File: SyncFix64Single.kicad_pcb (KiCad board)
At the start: 2 copper layers, 27.9 x 12.7 mm, 15 parts, among them J1 PWR, J2 Video, Q1 BSS138, Q2 BSS138, U1 LM1881, U2 AMS1117-50

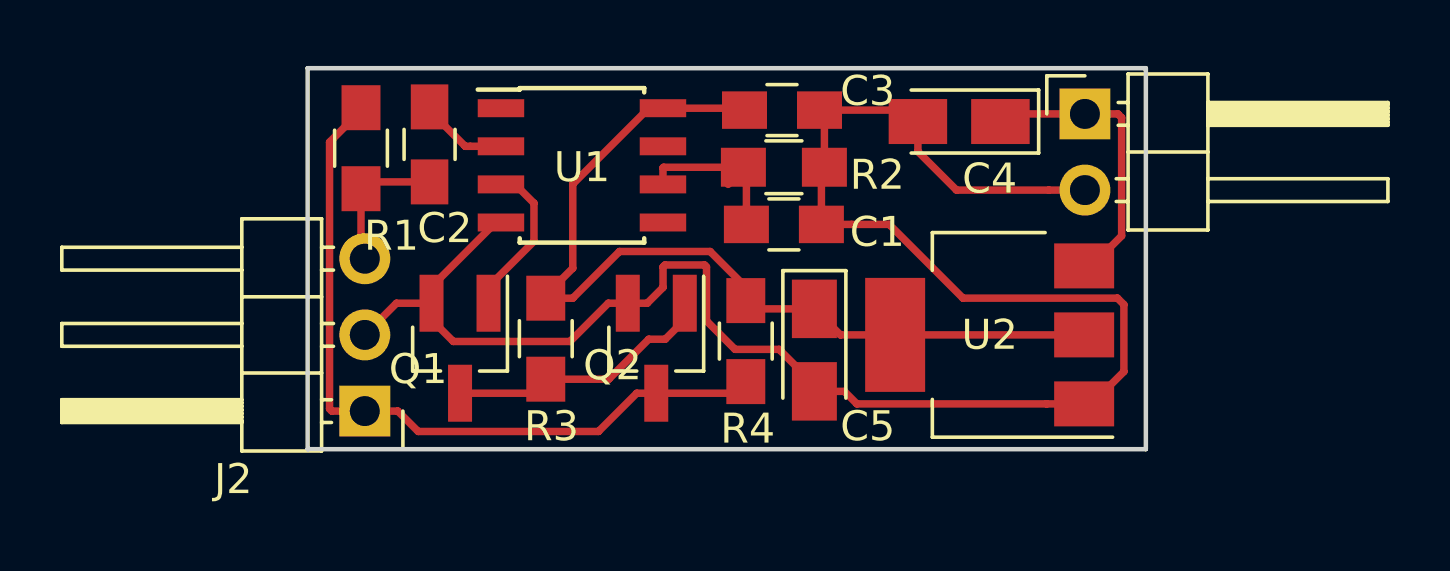
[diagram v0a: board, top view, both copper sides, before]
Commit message: Minor fixes.
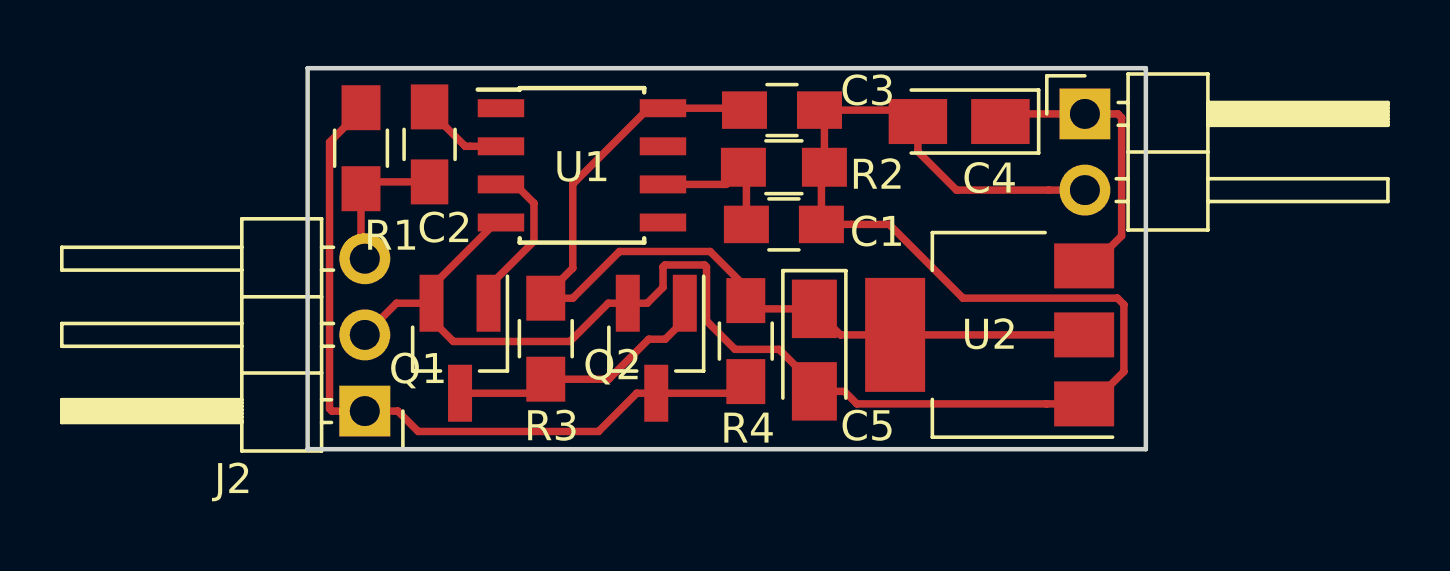
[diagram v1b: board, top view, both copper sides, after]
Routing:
- net Net-(C1-Pad1): track 5.96 -> 5.01 mm
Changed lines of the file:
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@@
     (thickness 1.6)
     (drawings 6)
-    (tracks 108)
+    (tracks 106)
     (zones 0)
     (modules 15)
@@
   (gr_line (start 57.15 27.94) (end 57.15 40.64) (angle 90) (layer Edge.Cuts) (width 0.15))
   (gr_line (start 29.21 27.94) (end 29.21 40.64) (angle 90) (layer Edge.Cuts) (width 0.15))
-  (segment (start 43.735 31.242) (end 41.0755 31.242) (width 0.25) (layer F.Cu) (net 1))
-  (segment (start 41.0755 31.242) (end 41.054 31.2635) (width 0.25) (layer F.Cu) (net 1))
-  (segment (start 41.054 31.2635) (end 41.054 31.8135) (width 0.25) (layer F.Cu) (net 1))
+  (segment (start 41.054 31.8135) (end 43.1635 31.8135) (width 0.25) (layer F.Cu) (net 1))
+  (segment (start 43.1635 31.8135) (end 43.735 31.242) (width 0.25) (layer F.Cu) (net 1))
   (segment (start 43.835 33.147) (end 43.835 31.342) (width 0.25) (layer F.Cu) (net 1))
   (segment (start 43.835 31.342) (end 43.735 31.242) (width 0.25) (layer F.Cu) (net 1))
   (segment (start 43.6715 33.301) (end 43.7715 33.401) (width 0.25) (layer F.Cu) (net 1))
-  (segment (start 43.227 31.8135) (end 43.6715 31.369) (width 0.25) (layer F.Cu) (net 1) (status 30))
   (segment (start 49.552 29.718) (end 49.552 30.718) (width 0.25) (layer F.Cu) (net 2))
   (segment (start 49.552 30.718) (end 50.838 32.004) (width 0.25) (layer F.Cu) (net 2))
